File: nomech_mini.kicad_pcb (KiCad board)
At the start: 2 copper layers, 100 x 80 mm, 10 parts

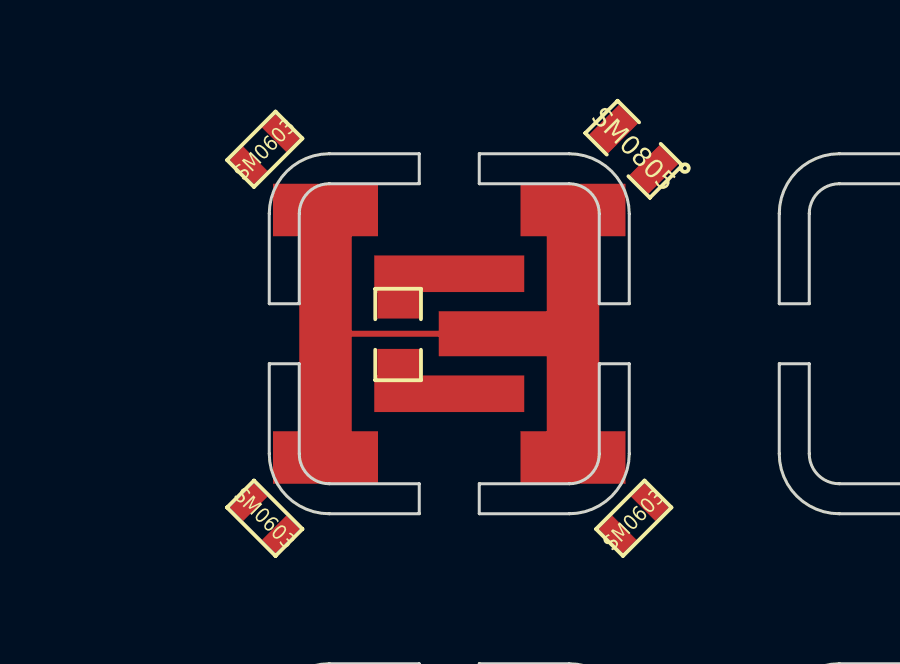
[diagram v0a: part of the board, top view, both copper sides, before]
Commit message: working mainly on LEDs
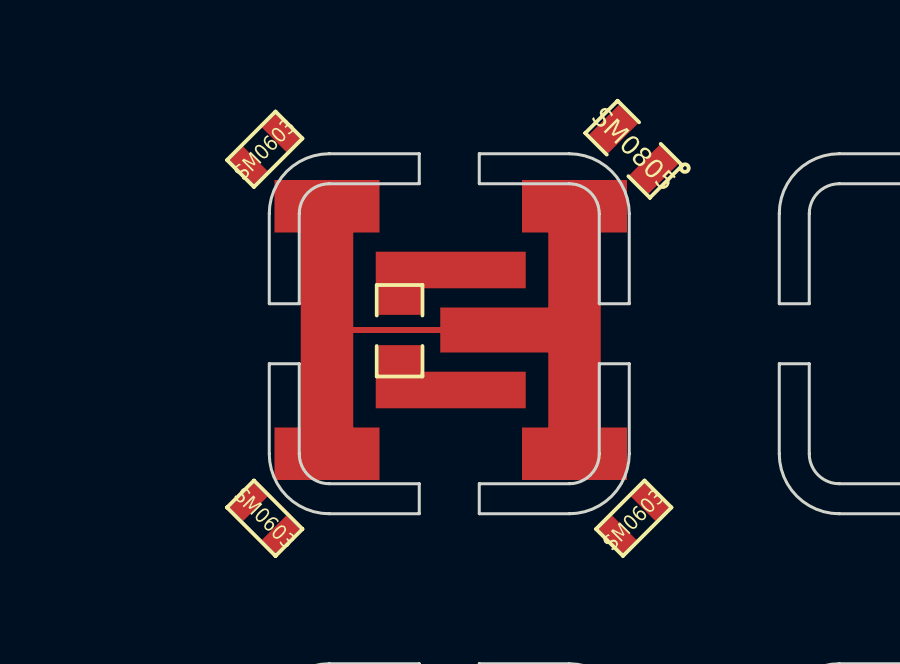
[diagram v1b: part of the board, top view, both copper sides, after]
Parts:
- moved cap-electrode_10mm 0.13 mm to (113.3, 89.1)
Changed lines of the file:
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@@
     (22 B.Mask user)
     (23 F.Mask user)
-    (24 Dwgs.User user hide)
+    (24 Dwgs.User user)
     (25 Cmts.User user)
     (26 Eco1.User user)
@@
   )
   (module cap-electrode_10mm (layer Front)
-    (at 113.25 89.25)
+    (at 113.3 89.125)
     (attr smd)
     (fp_text reference cap-electrode_10mm (at 0.1 6.4) (layer B.SilkS)
